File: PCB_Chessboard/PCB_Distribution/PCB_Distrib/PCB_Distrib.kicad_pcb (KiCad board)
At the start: 2 copper layers, 50 x 50 mm, 11 parts

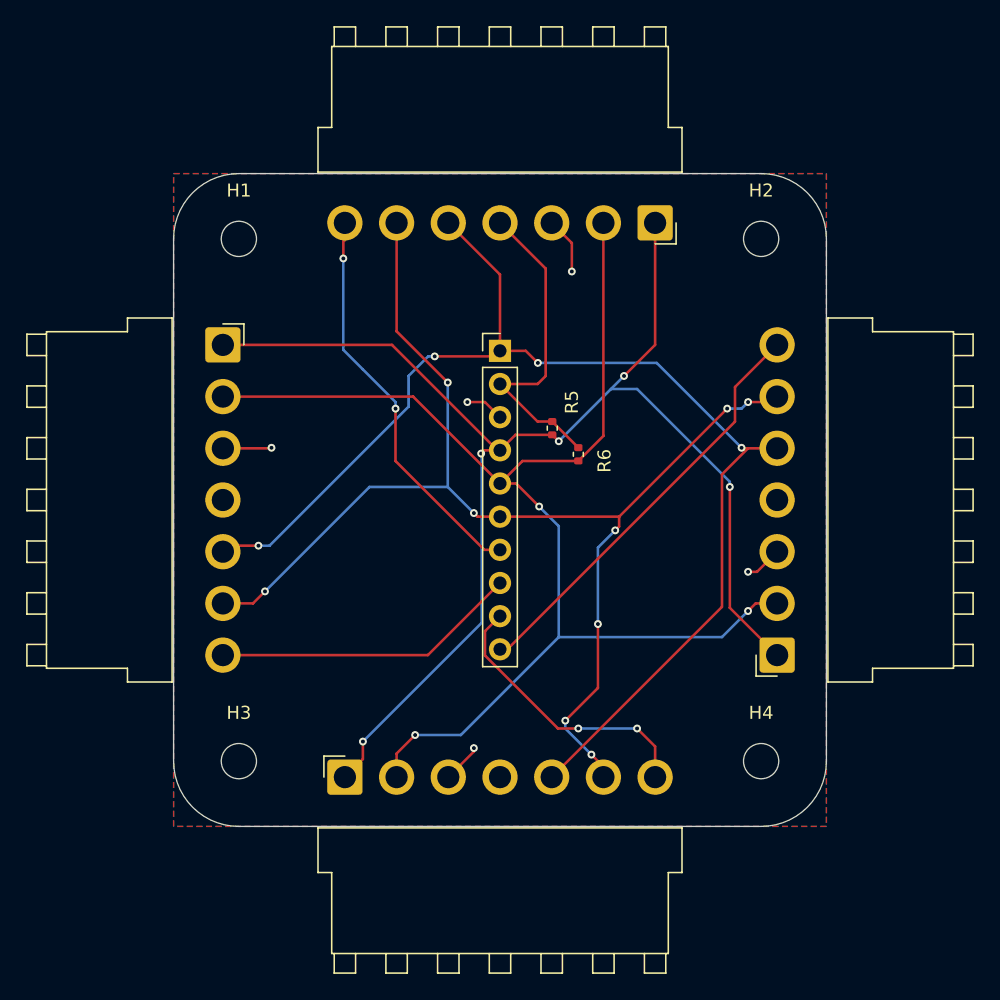
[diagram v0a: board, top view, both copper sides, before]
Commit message: update pcb
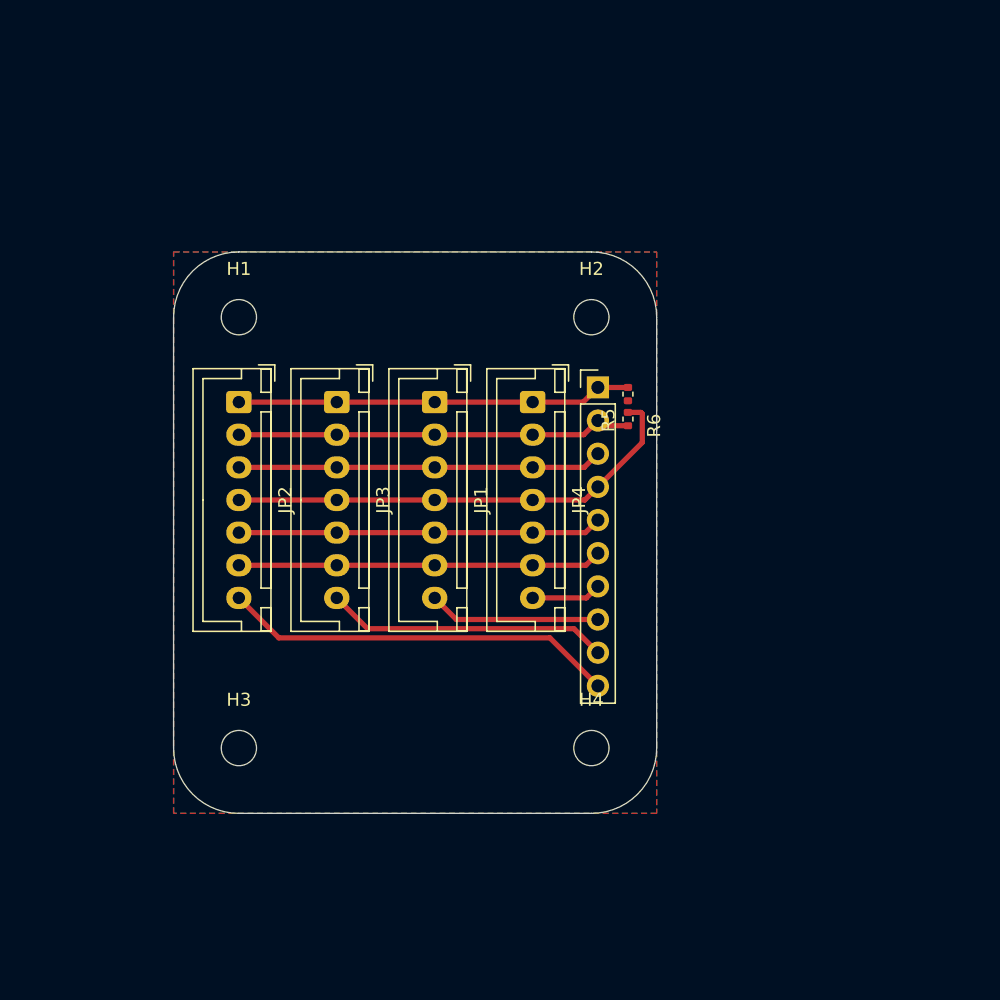
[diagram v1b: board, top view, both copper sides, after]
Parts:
- JP1, JP2, JP3, JP4: footprint Connector_JST:JST_VH_B7PS-VH_1x07_P3.96mm_Horizontal -> Connector_JST:JST_XH_B7B-XH-A_1x07_P2.50mm_Vertical
- moved JP3 28.7 mm to (112.5, 117.5), turned to -90 degrees
- moved JP4 26.9 mm to (127.5, 117.5), turned to -90 degrees
- moved JP1 21.8 mm to (120.0, 117.5), turned to -90 degrees
- moved H2 14.3 mm to (132.0, 111.0)
- moved H4 13.0 mm to (132.0, 144.0)
- moved JRasp1 8.01 mm to (132.5, 116.4)
- moved R5 6.36 mm to (134.8, 116.9), turned to 90 degrees
- moved H1 6.00 mm to (105.0, 111.0)
- moved R6 4.66 mm to (134.8, 118.8)
- moved JP2 4.55 mm to (105.0, 117.5)
- moved H3 1.00 mm to (105.0, 144.0)
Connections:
- JRasp1 pad 1: +5V -> SDA
- JRasp1 pad 10: GPIO22 -> GPIO04
- JRasp1 pad 2: +3.3V -> SCL
- JRasp1 pad 4: SDA -> +3.3V
- JRasp1 pad 5: SCL -> +5V
- JRasp1 pad 7: GPIO17 -> GPIO22
- JRasp1 pad 8: GPIO04 -> GPIO17
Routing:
- net SDA: track 107.1 -> 30.3 mm, vias 5 -> 0
- net SCL: track 99.8 -> 30.4 mm, vias 3 -> 0
- net +5V: track 96.1 -> 27.9 mm, vias 4 -> 0
- net LED.DIN: track 95.6 -> 27.9 mm, vias 9 -> 0
- net GPIO22: track 32.4 -> 5.37 mm
- net GPIO17: track 32.1 -> 13.2 mm, vias 2 -> 0
- net GND: track 17.0 -> 27.9 mm, vias 5 -> 0
- net +3.3V: track 26.2 -> 36.1 mm
- net GPIO04: track 23.5 -> 30.3 mm
- net GPIO27: track 21.8 -> 21.7 mm, vias 2 -> 0
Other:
- board size 50 x 50 mm -> 37 x 43 mm
